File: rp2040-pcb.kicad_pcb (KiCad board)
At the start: 2 copper layers, 23.2 x 51.2 mm, 43 parts, among them J1 Conn_01x20_Male, J2 Conn_01x20_Male, J3 TYPE-C-31-M-12, SW1 SW_Push, SW2 SW_Push, U1 RP2040, U2 TPS54202DDC, U3 W25Q128JVSIQ, Y1 12 MHz

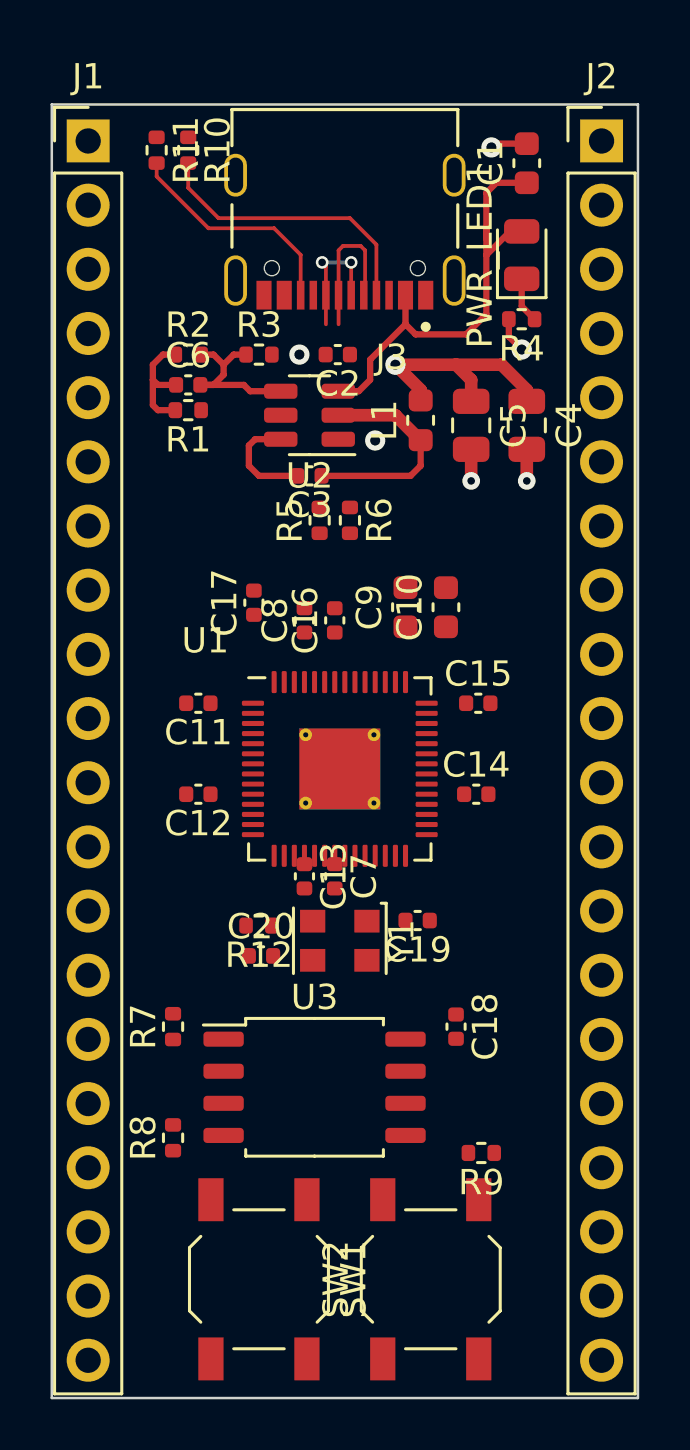
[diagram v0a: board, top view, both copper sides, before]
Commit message: Routed even more
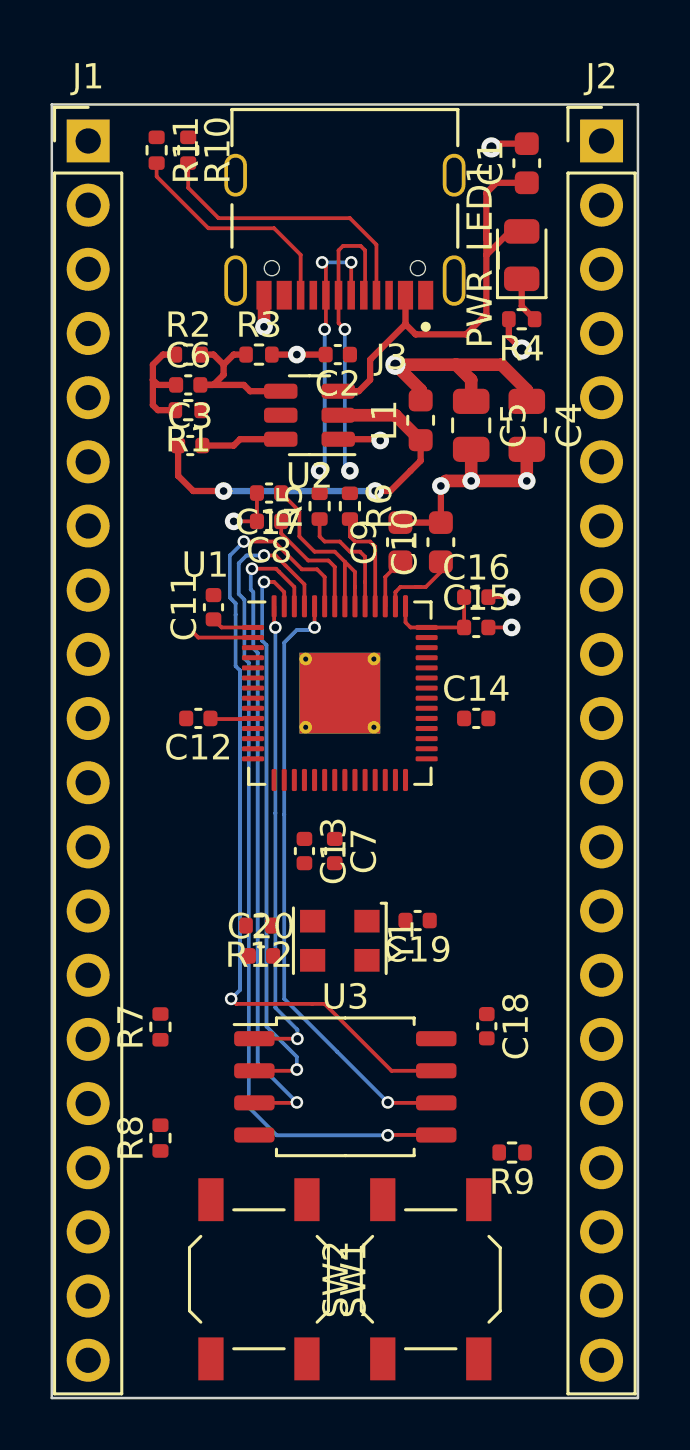
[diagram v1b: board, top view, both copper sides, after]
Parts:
- moved C16 5.68 mm to (106.8, 96.8), turned to 0 degrees
- moved C3 4.87 mm to (95.5, 90.8), turned to 0 degrees
- moved C17 4.38 mm to (98.6, 92.7), turned to 180 degrees
- moved C8 4.16 mm to (98.6, 93.8), turned to 180 degrees
- moved C11 3.85 mm to (96.4, 97.2), turned to 90 degrees
- moved C15 3.00 mm to (106.8, 98.0)
- moved C12 3.00 mm to (95.8, 101.6)
- moved C14 3.00 mm to (106.8, 101.6)
- moved U1 3.00 mm to (101.4, 100.6)
- moved C9 2.58 mm to (103.8, 94.6)
- moved C10 2.58 mm to (105.4, 94.6)
- moved C18 1.22 mm to (107.2, 113.8)
- moved R9 1.22 mm to (108.2, 118.8)
- moved U3 1.22 mm to (101.6, 116.2)
- moved C13 1.00 mm to (100.0, 106.8)
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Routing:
- net QSPI SD0: track 0.00 -> 33.7 mm, vias 0 -> 2
- net QSPI SD3: track 0.00 -> 32.9 mm, vias 0 -> 2
- net QSPI SD2: track 0.00 -> 26.5 mm, vias 0 -> 2
- net QSPI CLK: track 0.00 -> 24.2 mm, vias 0 -> 2
- net QSPI SD1: track 0.00 -> 23.1 mm, vias 0 -> 2
- net +3.3V: track 9.59 -> 28.8 mm
- net QSPI CS: track 0.00 -> 19.2 mm, vias 0 -> 2
- net GND: track 5.37 -> 20.8 mm, vias 4 -> 11
- net Net-(C3-Pad1): track 8.77 -> 16.0 mm, vias 0 -> 2
- net +1V1: track 0.00 -> 6.72 mm
- net USB D-: track 5.92 -> 11.8 mm, vias 0 -> 2
- net USB D+: track 4.96 -> 10.8 mm, vias 2 -> 4
- net /N_USB_D+: track 0.00 -> 4.78 mm
- net /N_USB_D-: track 0.00 -> 4.22 mm
- net GPIO0: track 0.00 -> 2.45 mm
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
